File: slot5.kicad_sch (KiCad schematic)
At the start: 1 part

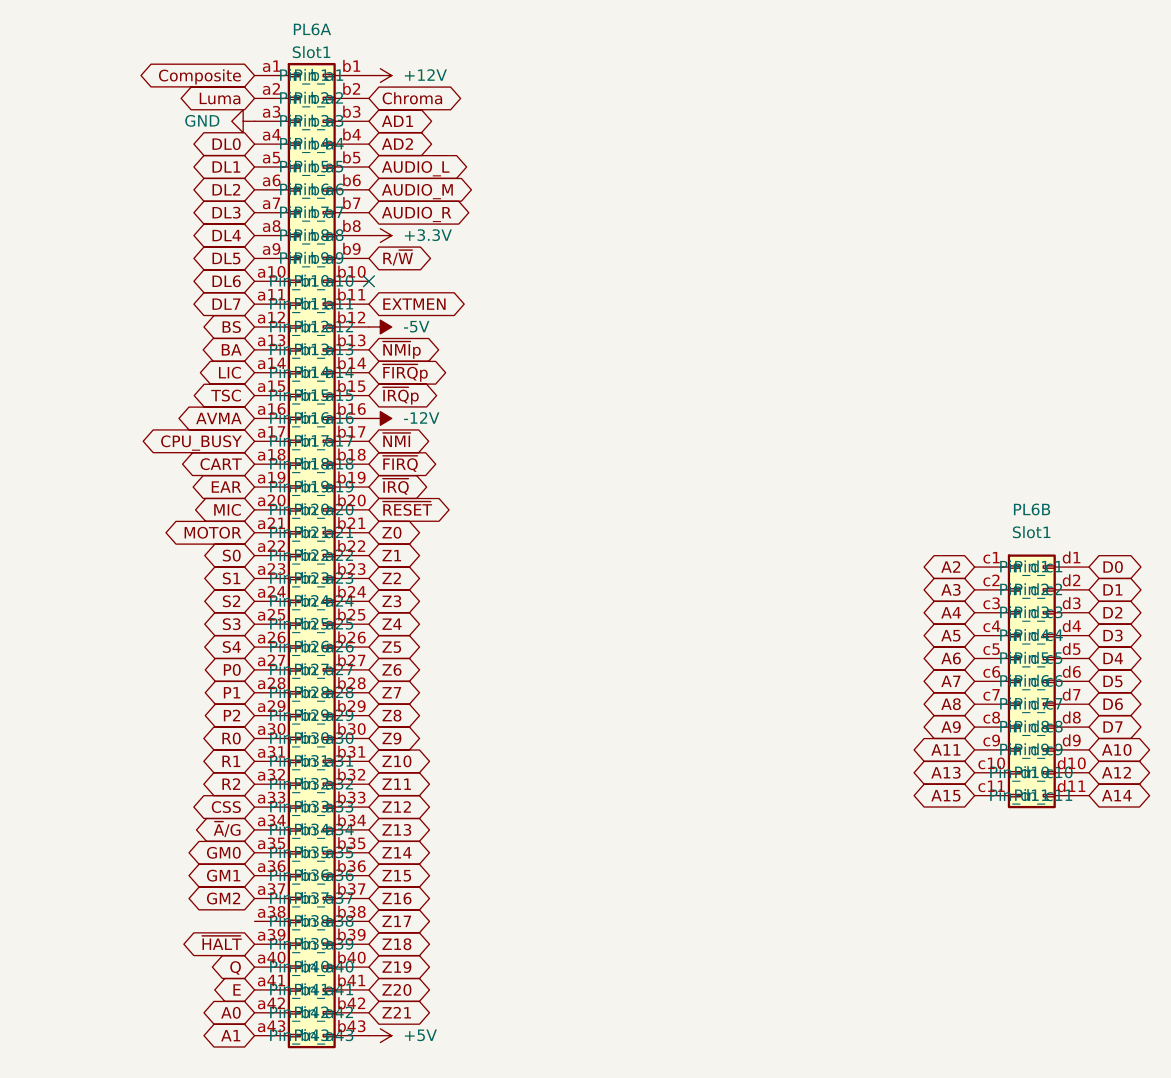
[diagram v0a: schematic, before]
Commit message: board layout
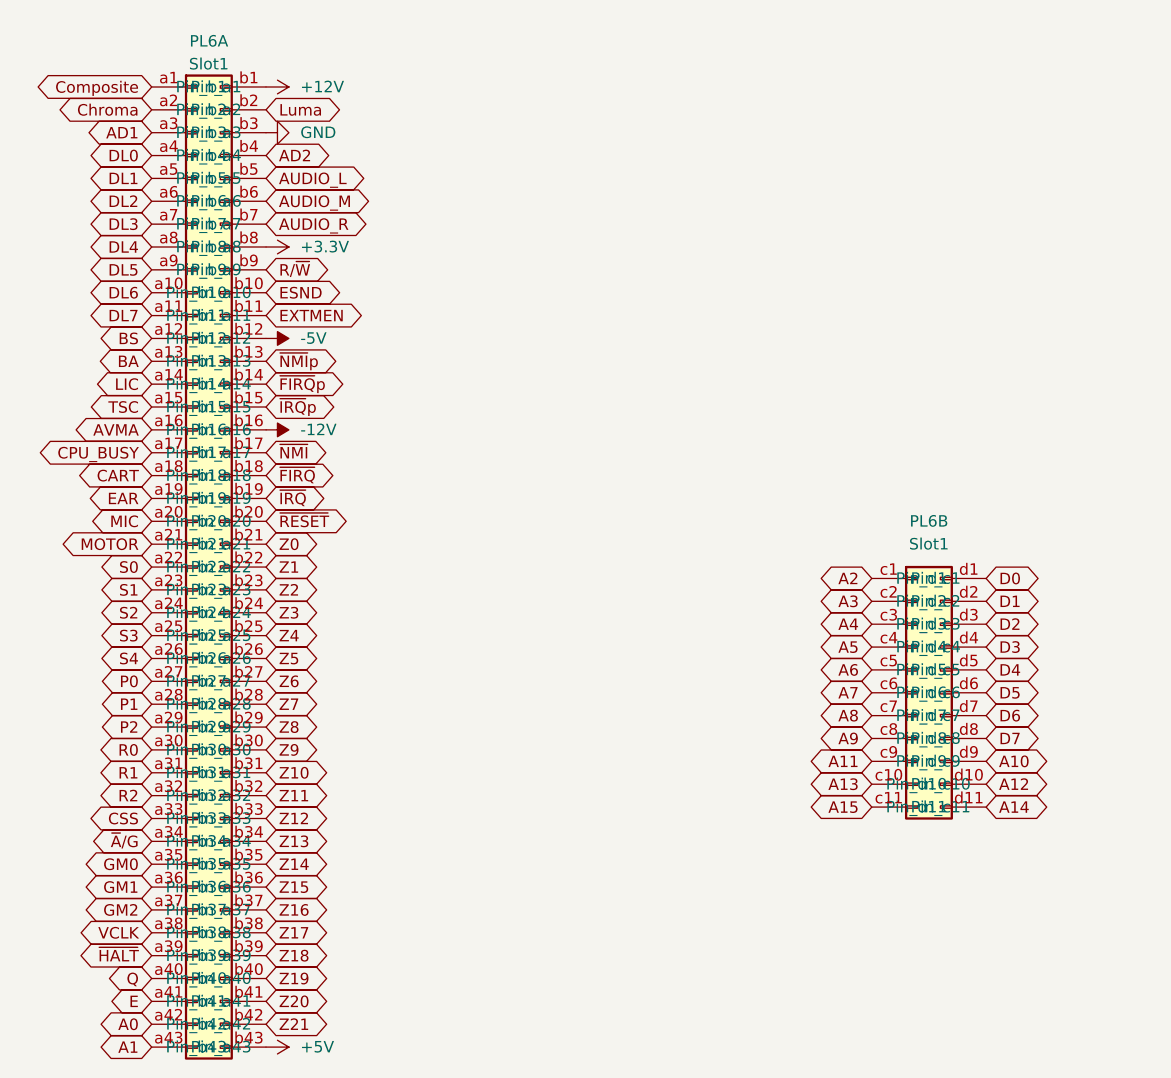
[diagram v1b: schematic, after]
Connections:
- net AD1: now also PL6.a3 (Pin_a3); no longer PL6.b3 (Pin_b3)
- net Chroma: now also PL6.a2 (Pin_a2); no longer PL6.b2 (Pin_b2)
- net GND: now also PL6.b3 (Pin_b3); no longer PL6.a3 (Pin_a3)
- net Luma: now also PL6.b2 (Pin_b2); no longer PL6.a2 (Pin_a2)
- net VCLK: now reaches PL6.a38 (Pin_a38)
- net ESND: now reaches PL6.b10 (Pin_b10)
- no-connect marks 1 -> 0
